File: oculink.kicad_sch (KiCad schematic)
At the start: 11 parts, among them J4 OCuLink_x4_Amphenol_G14A42121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, U2 MAX3373EEKA+

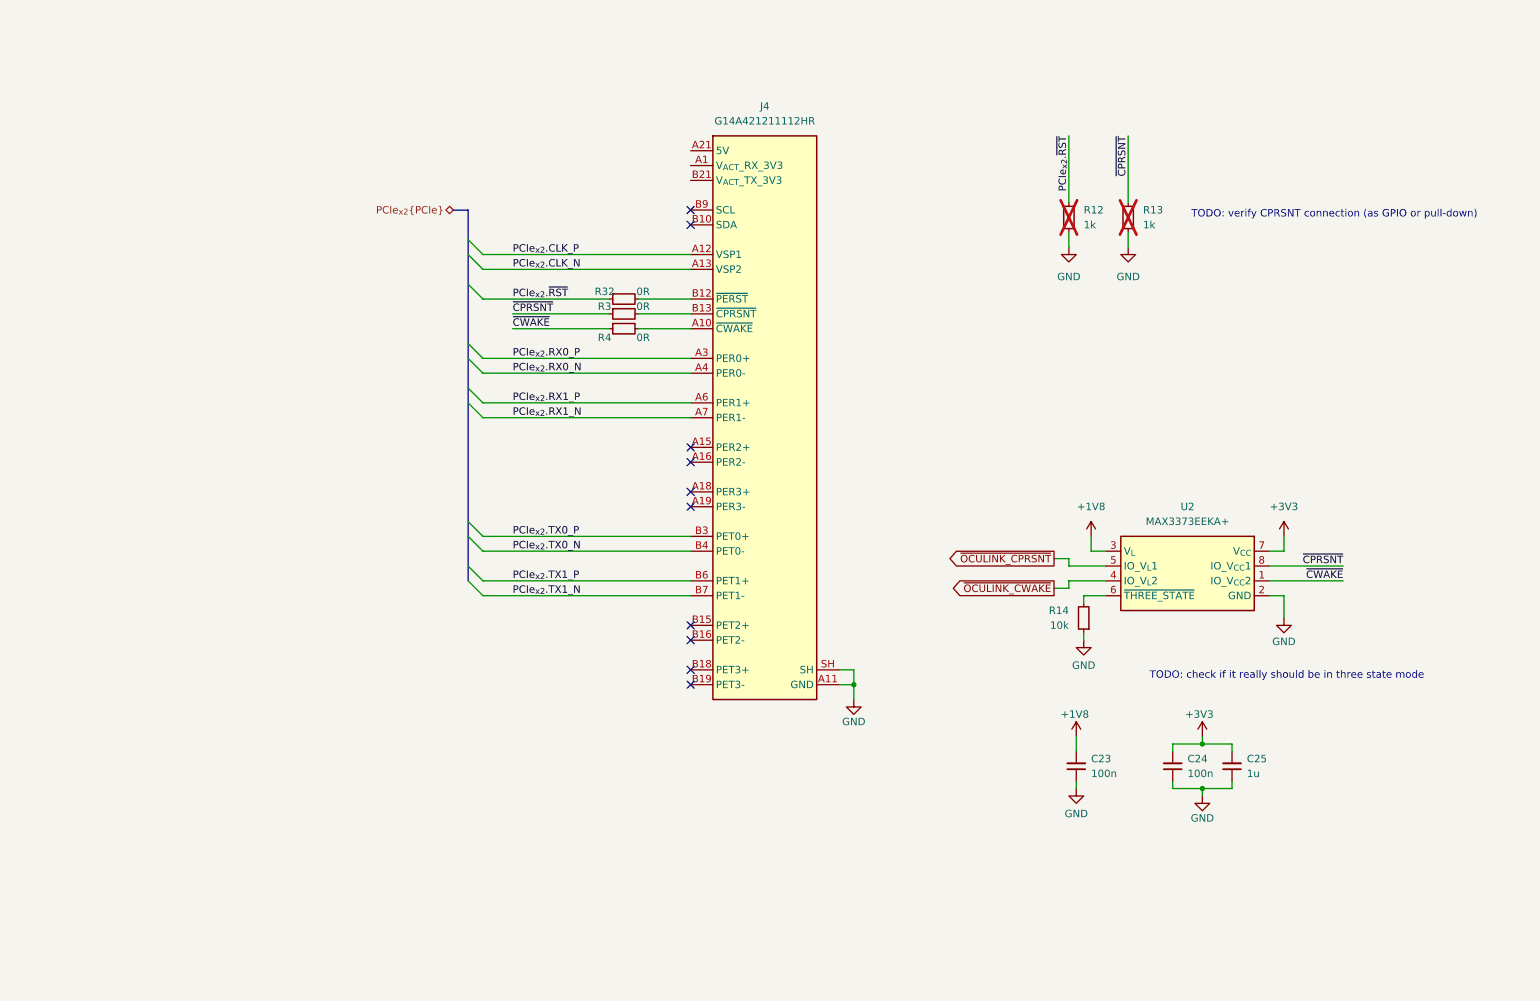
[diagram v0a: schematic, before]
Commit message: [#100765] Update schematic
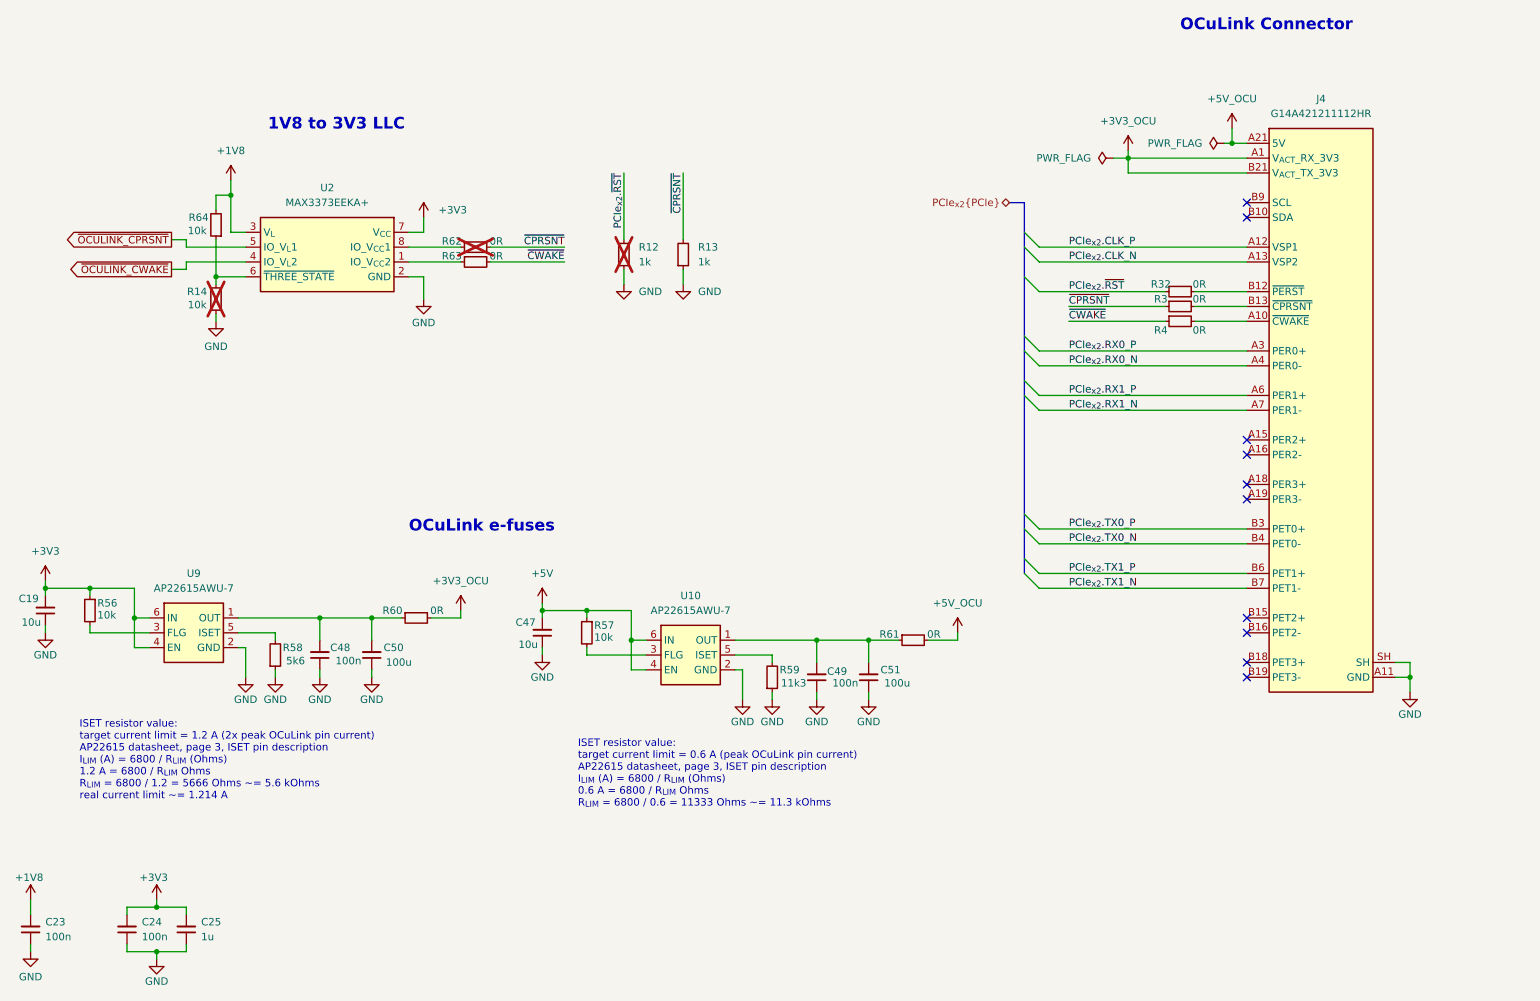
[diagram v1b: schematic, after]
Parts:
- added C19, C47: C_10u_0402, antmicro-footprints:C_0402_1005Metric, symbol antmicroCapacitors0402:C_10u_0402
- added C48, C49: C_100n_0402, antmicro-footprints:C_0402_1005Metric, symbol antmicroCapacitors0402:C_100n_0402
- added C50, C51: C_100u_0805, antmicro-footprints:C_0805_2012Metric, symbol antmicroCapacitorsmisc:C_100u_0805
- added R56, R57, R64: R_10k_0402, antmicro-footprints:R_0402_1005Metric, symbol antmicroResistors0402:R_10k_0402
- added R58: R_5k6_0402, antmicro-footprints:R_0402_1005Metric, symbol antmicroResistors0402:R_5k6_0402
- added R59: R_11k3_0402, antmicro-footprints:R_0402_1005Metric, symbol antmicroResistors0402:R_11k3_0402
- added R60, R61, R62, R63: R_0R_0402, antmicro-footprints:R_0402_1005Metric, symbol antmicroResistors0402:R_0R_0402
- added U10, U9: (no value), antmicro-footprints:TSOT23-6, symbol antmicroPMICPowerDistributionSwitchesLoadDrivers:AP22615A_TSOT26
- R13: now fitted
- R14: now not fitted
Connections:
- net +1V8: now also R64.2
- net +3V3: now also C19.2, R56.1, U9.4 (EN), U9.6 (IN)
- net GND: now also C19.1, C47.1, C48.1, C49.1, C50.1, C51.1, R58.1, R59.1, U10.2 (GND), U9.2 (GND)
- net ~{CPRSNT}: now also R62.2; no longer U2.8 (IO_V_{CC}1)
- net ~{CWAKE}: now also R63.2; no longer U2.1 (IO_V_{CC}2)
- net at R14.2, U2.6 (~{THREE_STATE}): now also R64.1
- net +3V3_OCU: now reaches J4.A1 (V_{ACT}_RX_3V3)
- net +3V3_OCU: now also J4.B21 (V_{ACT}_TX_3V3), R60.2
- net +5V_OCU: now reaches J4.A21 (5V), J4.B1 (5V)
- net +5V_OCU: now also R61.2
- new net: C48.2, C50.2, R60.1, U9.1 (OUT)
- new net: C49.2, C51.2, R61.1, U10.1 (OUT)
- new net: R58.2, U9.5 (ISET)
- new net: R59.2, U10.5 (ISET)
- new net: R56.2, U9.3 (FLG)
- new net: R63.1, U2.1 (IO_V_{CC}2)
- new net: R62.1, U2.8 (IO_V_{CC}1)
- new net: R57.2, U10.3 (FLG)
- new net +5V: C47.2, R57.1, U10.4 (EN), U10.6 (IN)
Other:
- note added: "1V8 to 3V3 LLC"
- note added: "ISET resistor value: target current limit = 0.6 A (peak OCuLink pin current) AP22615 datasheet, page 3, ISET pin description I_{LIM} (A) = 6800 / R_{LIM} (Ohms) 0.6 A = 6800 / R_{LIM} Ohms R_{LIM} = 6800 / 0.6 = 11333 Ohms ~= 11.3 kOhms"
- note added: "ISET resistor value: target current limit = 1.2 A (2x peak OCuLink pin current) AP22615 datasheet, page 3, ISET pin description I_{LIM} (A) = 6800 / R_{LIM} (Ohms) 1.2 A = 6800 / R_{LIM} Ohms R_{LIM} = 6800 / 1.2 = 5666 Ohms ~= 5.6 kOhms real current limit ~= 1.214 A"
- note added: "OCuLink Connector"
- note added: "OCuLink e-fuses"
- note removed: "TODO: check if it really should be in three state mode"
- note removed: "TODO: verify CPRSNT connection (as GPIO or pull-down)"
- moved on the sheet: C23, C24, C25, J4, R12, R3, R32, R4, U2
